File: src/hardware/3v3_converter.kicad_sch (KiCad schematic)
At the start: 3 parts

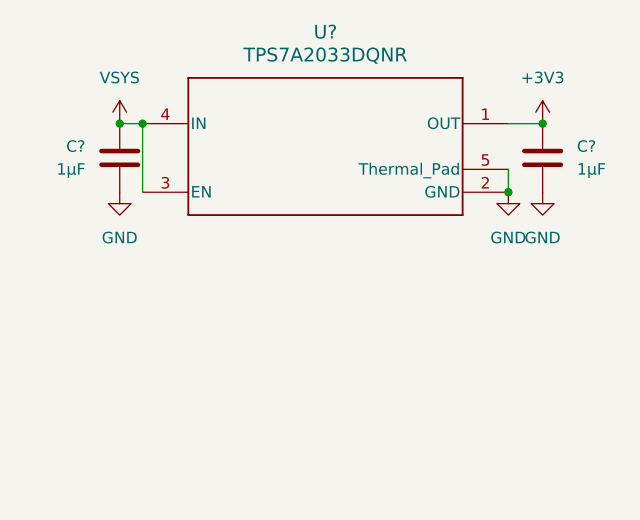
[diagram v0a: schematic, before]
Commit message: Created Power Diagram
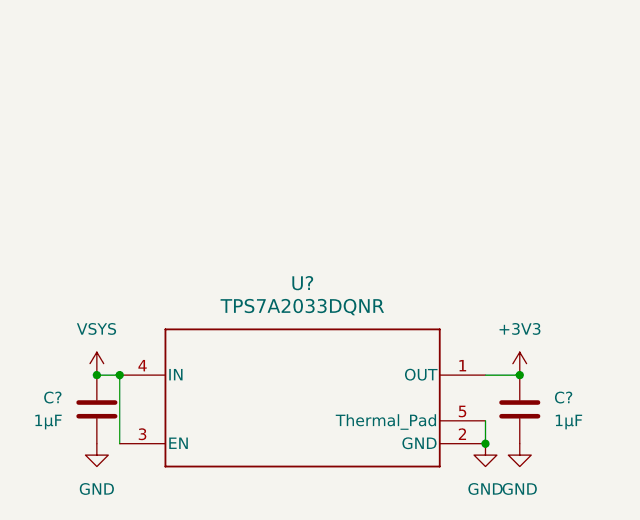
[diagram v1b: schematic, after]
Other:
- moved on the sheet: C?, U?
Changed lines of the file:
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@@
 	)
 	(junction
-		(at 172.72 81.28)
+		(at 170.18 109.22)
 		(diameter 0)
 		(color 0 0 0 0)
 	)
 	(junction
-		(at 176.53 73.66)
+		(at 173.99 101.6)
 		(diameter 0)
 		(color 0 0 0 0)
 	)
 	(junction
-		(at 132.08 73.66)
+		(at 129.54 101.6)
 		(diameter 0)
 		(color 0 0 0 0)
 	)
 	(junction
-		(at 129.54 73.66)
+		(at 127 101.6)
 		(diameter 0)
 		(color 0 0 0 0)
@@
 	(wire
 		(pts
-			(xy 172.72 73.66) (xy 176.53 73.66)
+			(xy 170.18 101.6) (xy 173.99 101.6)
 		)
 		(stroke
@@
 	(wire
 		(pts
-			(xy 172.72 78.74) (xy 172.72 81.28)
+			(xy 170.18 106.68) (xy 170.18 109.22)
 		)
 		(stroke
@@
 	(wire
 		(pts
-			(xy 129.54 73.66) (xy 132.08 73.66)
+			(xy 127 101.6) (xy 129.54 101.6)
 		)
 		(stroke
@@
 	(wire
 		(pts
-			(xy 132.08 73.66) (xy 132.08 81.28)
+			(xy 129.54 101.6) (xy 129.54 109.22)
 		)
 		(stroke
@@
 	(symbol
 		(lib_id "TPS7A2033DQNR:TPS7A2033DQNR")
-		(at 132.08 73.66 0)
+		(at 129.54 101.6 0)
 		(unit 1)
 		(exclude_from_sim no)
@@
 		(fields_autoplaced yes)
 		(property "Reference" "U?"
-			(at 152.4 63.5 0)
+			(at 149.86 91.44 0)
 			(effects
 				(font
@@
 		)
 		(property "Value" "TPS7A2033DQNR"
-			(at 152.4 66.04 0)
+			(at 149.86 93.98 0)
 			(effects
 				(font
@@
 		)
 		(property "Footprint" "DQN0004A-MFG"
-			(at 132.08 73.66 0)
+			(at 129.54 101.6 0)
 			(effects
 				(font
@@
 		)
 		(property "Datasheet" "https://www.ti.com/lit/gpn/tps7a20"
-			(at 132.08 73.66 0)
+			(at 129.54 101.6 0)
 			(effects
 				(font
@@
 		)
 		(property "Description" ""
-			(at 132.08 73.66 0)
+			(at 129.54 101.6 0)
 			(effects
 				(font
@@
 	(symbol
 		(lib_id "power:GND")
-		(at 176.53 81.28 0)
+		(at 173.99 109.22 0)
 		(unit 1)
 		(exclude_from_sim no)
@@
 		(fields_autoplaced yes)
 		(property "Reference" "#PWR0395"
-			(at 176.53 87.63 0)
+			(at 173.99 115.57 0)
 			(effects
 				(font
@@
 		)
 		(property "Value" "GND"
-			(at 176.53 86.36 0)
-			(effects
-				(font
-					(size 1.27 1.27)
-				)
-			)
-		)
-		(property "Footprint" ""
-			(at 176.53 81.28 0)
+			(at 173.99 114.3 0)
+			(effects
+				(font
+					(size 1.27 1.27)
+				)
+			)
+		)
+		(property "Footprint" ""
+			(at 173.99 109.22 0)
 			(effects
 				(font
@@
 		)
 		(property "Datasheet" ""
-			(at 176.53 81.28 0)
+			(at 173.99 109.22 0)
 			(effects
 				(font
@@
 		)
 		(property "Description" "Power symbol creates a global label with name \"GND\" , ground"
-			(at 176.53 81.28 0)
+			(at 173.99 109.22 0)
 			(effects
 				(font
@@
 	(symbol
 		(lib_id "Device:C")
-		(at 129.54 77.47 0)
+		(at 127 105.41 0)
 		(mirror y)
 		(unit 1)
@@
 		(fields_autoplaced yes)
 		(property "Reference" "C?"
-			(at 125.73 76.1999 0)
+			(at 123.19 104.1399 0)
 			(effects
 				(font
@@
 		)
 		(property "Value" "1µF"
-			(at 125.73 78.7399 0)
+			(at 123.19 106.6799 0)
 			(effects
 				(font
@@
 		)
 		(property "Footprint" ""
-			(at 128.5748 81.28 0)
+			(at 126.0348 109.22 0)
 			(effects
 				(font
@@
 		)
 		(property "Datasheet" "~"
-			(at 129.54 77.47 0)
+			(at 127 105.41 0)
 			(effects
 				(font
@@
 		)
 		(property "Description" "Unpolarized capacitor"
-			(at 129.54 77.47 0)
+			(at 127 105.41 0)
 			(effects
 				(font
@@
 	(symbol
 		(lib_id "power:LINE")
-		(at 129.54 73.66 0)
+		(at 127 101.6 0)
 		(unit 1)
 		(exclude_from_sim no)
@@
 		(fields_autoplaced yes)
 		(property "Reference" "#PWR0391"
-			(at 129.54 77.47 0)
+			(at 127 105.41 0)
 			(effects
 				(font
@@
 		)
 		(property "Value" "VSYS"
-			(at 129.54 68.58 0)
-			(effects
-				(font
-					(size 1.27 1.27)
-				)
-			)
-		)
-		(property "Footprint" ""
-			(at 129.54 73.66 0)
+			(at 127 96.52 0)
+			(effects
+				(font
+					(size 1.27 1.27)
+				)
+			)
+		)
+		(property "Footprint" ""
+			(at 127 101.6 0)
 			(effects
 				(font
@@
 		)
 		(property "Datasheet" ""
-			(at 129.54 73.66 0)
+			(at 127 101.6 0)
 			(effects
 				(font
@@
 		)
 		(property "Description" "Power symbol creates a global label with name \"LINE\""
-			(at 129.54 73.66 0)
+			(at 127 101.6 0)
 			(effects
 				(font
@@
 	(symbol
 		(lib_id "power:GND")
-		(at 172.72 81.28 0)
+		(at 170.18 109.22 0)
 		(unit 1)
 		(exclude_from_sim no)
@@
 		(fields_autoplaced yes)
 		(property "Reference" "#PWR0394"
-			(at 172.72 87.63 0)
+			(at 170.18 115.57 0)
 			(effects
 				(font
@@
 		)
 		(property "Value" "GND"
-			(at 172.72 86.36 0)
-			(effects
-				(font
-					(size 1.27 1.27)
-				)
-			)
-		)
-		(property "Footprint" ""
-			(at 172.72 81.28 0)
+			(at 170.18 114.3 0)
+			(effects
+				(font
+					(size 1.27 1.27)
+				)
+			)
+		)
+		(property "Footprint" ""
+			(at 170.18 109.22 0)
 			(effects
 				(font
@@
 		)
 		(property "Datasheet" ""
-			(at 172.72 81.28 0)
+			(at 170.18 109.22 0)
 			(effects
 				(font
@@
 		)
 		(property "Description" "Power symbol creates a global label with name \"GND\" , ground"
-			(at 172.72 81.28 0)
+			(at 170.18 109.22 0)
 			(effects
 				(font
@@
 	(symbol
 		(lib_id "power:+3V3")
-		(at 176.53 73.66 0)
+		(at 173.99 101.6 0)
 		(unit 1)
 		(exclude_from_sim no)
@@
 		(fields_autoplaced yes)
 		(property "Reference" "#PWR0393"
-			(at 176.53 77.47 0)
+			(at 173.99 105.41 0)
 			(effects
 				(font
@@
 		)
 		(property "Value" "+3V3"
-			(at 176.53 68.58 0)
-			(effects
-				(font
-					(size 1.27 1.27)
-				)
-			)
-		)
-		(property "Footprint" ""
-			(at 176.53 73.66 0)
+			(at 173.99 96.52 0)
+			(effects
+				(font
+					(size 1.27 1.27)
+				)
+			)
+		)
+		(property "Footprint" ""
+			(at 173.99 101.6 0)
 			(effects
 				(font
@@
 		)
 		(property "Datasheet" ""
-			(at 176.53 73.66 0)
+			(at 173.99 101.6 0)
 			(effects
 				(font
@@
 		)
 		(property "Description" "Power symbol creates a global label with name \"+3V3\""
-			(at 176.53 73.66 0)
+			(at 173.99 101.6 0)
 			(effects
 				(font
@@
 	(symbol
 		(lib_id "power:GND")
-		(at 129.54 81.28 0)
+		(at 127 109.22 0)
 		(unit 1)
 		(exclude_from_sim no)
@@
 		(fields_autoplaced yes)
 		(property "Reference" "#PWR0392"
-			(at 129.54 87.63 0)
+			(at 127 115.57 0)
 			(effects
 				(font
@@
 		)
 		(property "Value" "GND"
-			(at 129.54 86.36 0)
-			(effects
-				(font
-					(size 1.27 1.27)
-				)
-			)
-		)
-		(property "Footprint" ""
-			(at 129.54 81.28 0)
+			(at 127 114.3 0)
+			(effects
+				(font
+					(size 1.27 1.27)
+				)
+			)
+		)
+		(property "Footprint" ""
+			(at 127 109.22 0)
 			(effects
 				(font
@@
 		)
 		(property "Datasheet" ""
-			(at 129.54 81.28 0)
+			(at 127 109.22 0)
 			(effects
 				(font
@@
 		)
 		(property "Description" "Power symbol creates a global label with name \"GND\" , ground"
-			(at 129.54 81.28 0)
+			(at 127 109.22 0)
 			(effects
 				(font
@@
 	(symbol
 		(lib_id "Device:C")
-		(at 176.53 77.47 0)
+		(at 173.99 105.41 0)
 		(unit 1)
 		(exclude_from_sim no)
@@
 		(fields_autoplaced yes)
 		(property "Reference" "C?"
-			(at 180.34 76.1999 0)
+			(at 177.8 104.1399 0)
 			(effects
 				(font
@@
 		)
 		(property "Value" "1µF"
-			(at 180.34 78.7399 0)
+			(at 177.8 106.6799 0)
 			(effects
 				(font
@@
 		)
 		(property "Footprint" ""
-			(at 177.4952 81.28 0)
+			(at 174.9552 109.22 0)
 			(effects
 				(font
@@
 		)
 		(property "Datasheet" "~"
-			(at 176.53 77.47 0)
+			(at 173.99 105.41 0)
 			(effects
 				(font
@@
 		)
 		(property "Description" "Unpolarized capacitor"
-			(at 176.53 77.47 0)
-			(effects
-				(font
+			(at 173.99 105.41 0)
+			(effects
+				(font
